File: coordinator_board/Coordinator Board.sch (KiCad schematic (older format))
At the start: 26 parts, among them J1 Conn_01x04, J2 Conn_01x04, J3 Conn_01x04, J4 Conn_01x04, P4 SERIAL, SW1 Switch_SPDT_x2, SW2 Switch_DPST, U0 10118194, U1 LM3671, U3 ESP-12E, U4 DIY-OLED-0.96, U5 SF303GJ26, U6 CD40109B, U7 CD40109B

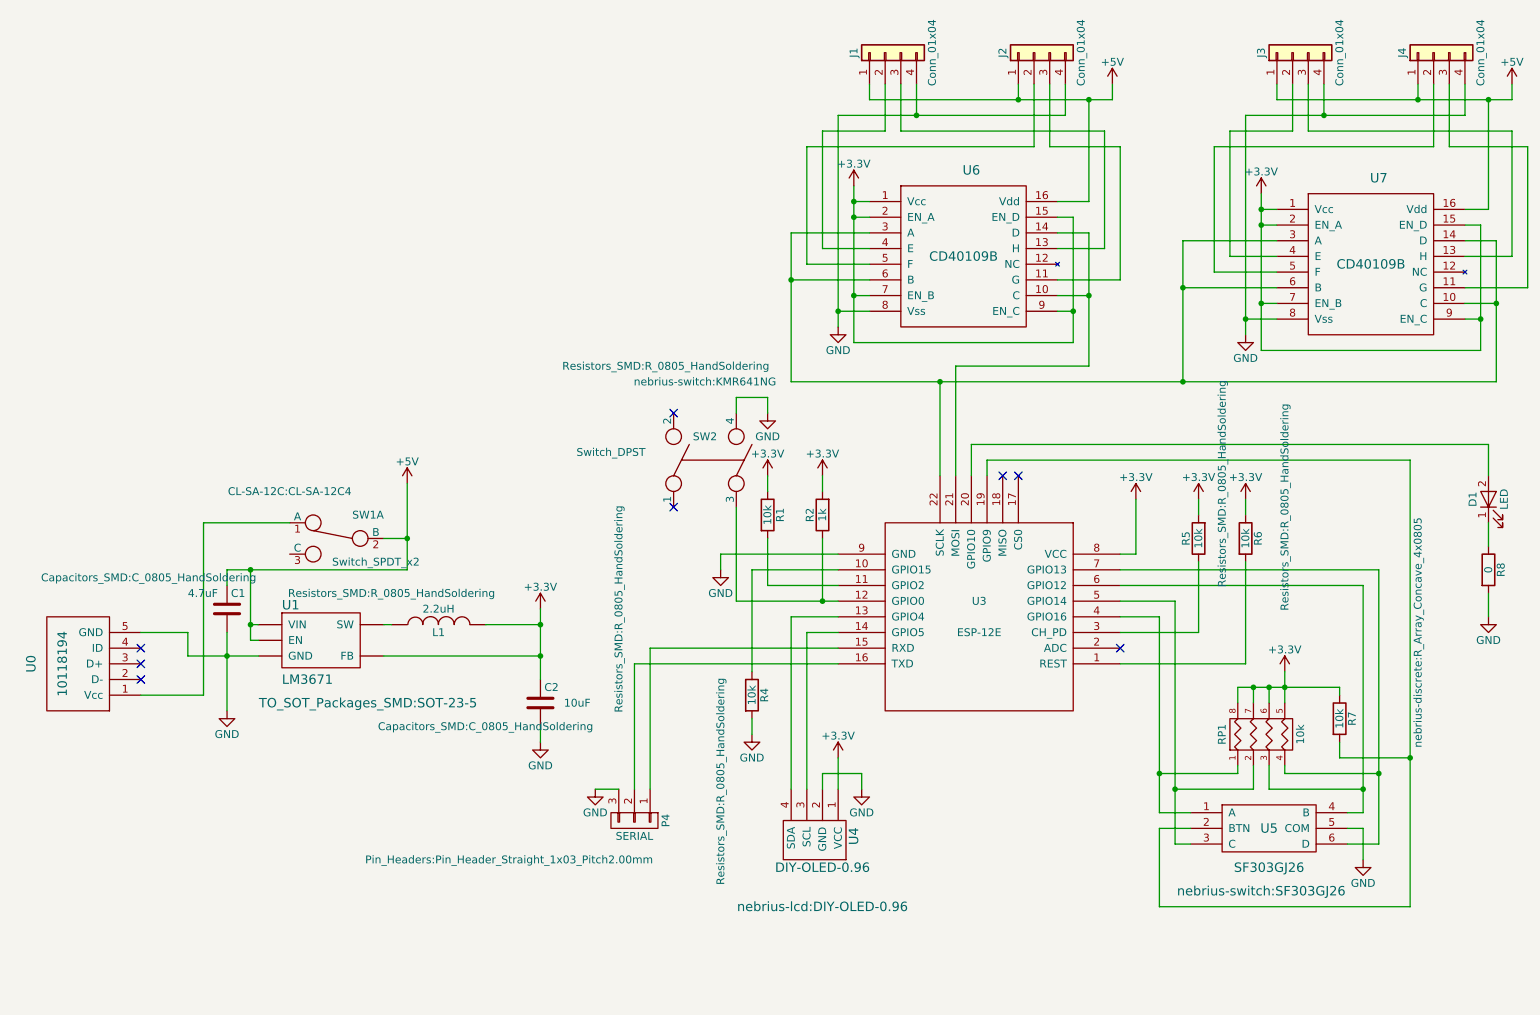
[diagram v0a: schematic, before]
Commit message: Finished most of the layout
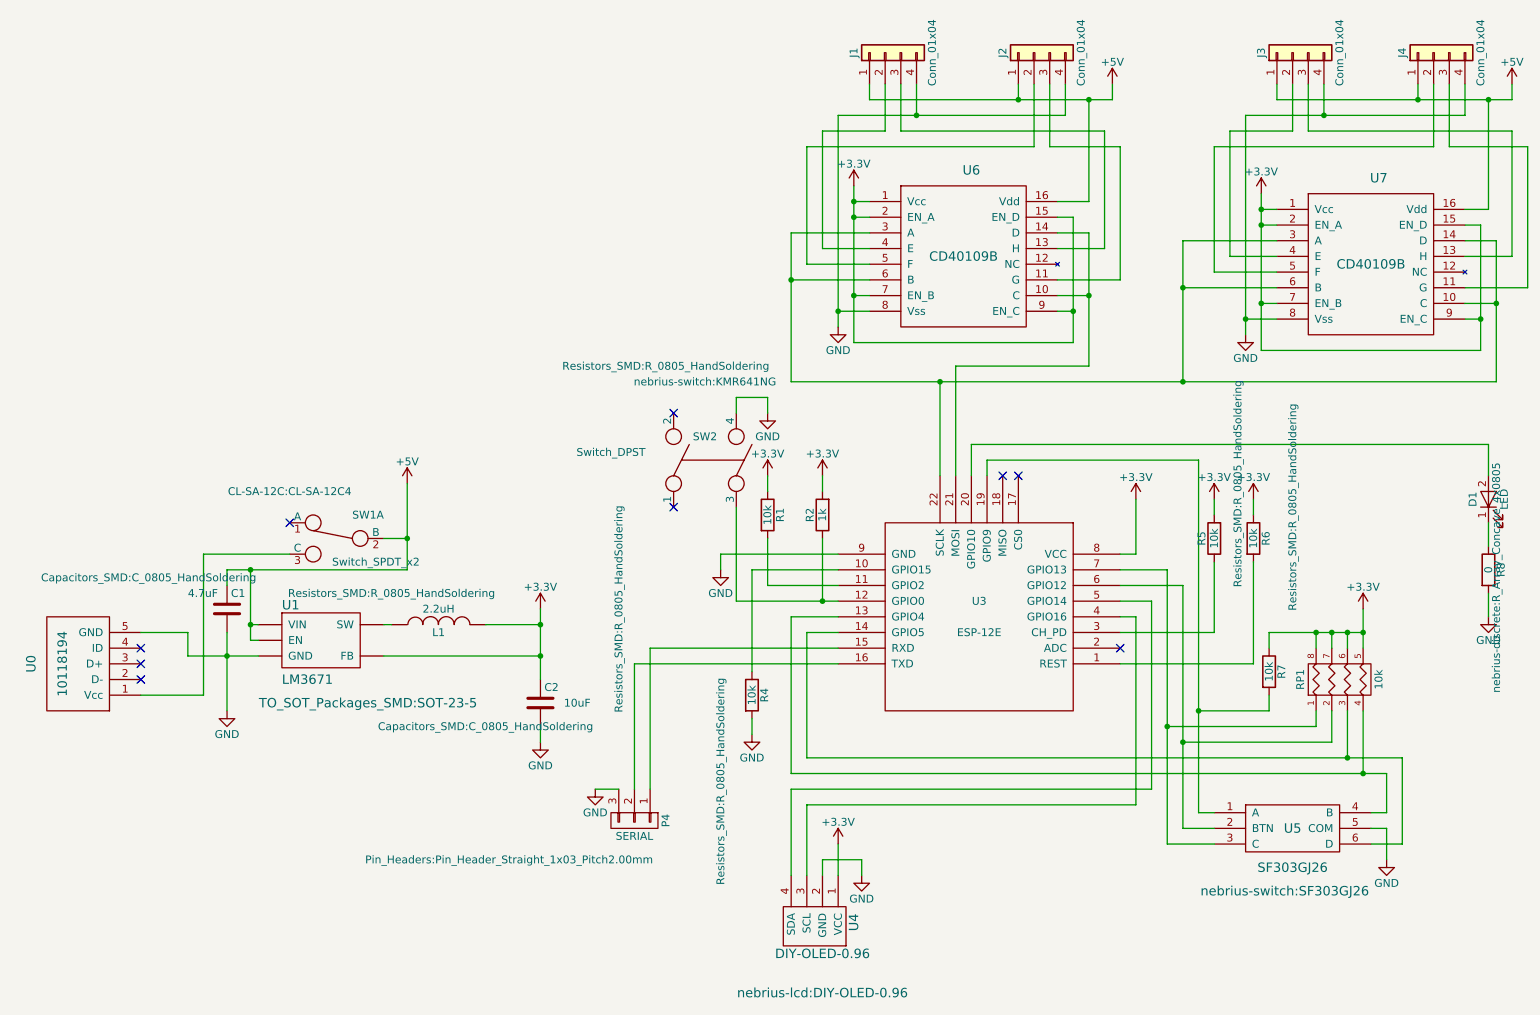
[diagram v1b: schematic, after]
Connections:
- net at SW1.1 (A): no longer U0.1 (Vcc)
- net at SW1.3 (C): now also U0.1 (Vcc)
- net at U3.13 (GPIO4): now also RP1.4 (P4), U5.4 (B); no longer U4.4 (SDA)
- net at U3.14 (GPIO5): now also RP1.3 (P3), U5.6 (D); no longer U4.3 (SCL)
- net at R7.2, U3.19 (GPIO9): now also U5.1 (A); no longer U5.2 (BTN)
- new net: U3.4 (GPIO16), U4.3 (SCL)
- new net: U3.5 (GPIO14), U4.4 (SDA)
- new net: RP1.2 (P2), U3.6 (GPIO12), U5.2 (BTN)
- new net: RP1.1 (P1), U3.7 (GPIO13), U5.3 (C)
- no-connect marks 8 -> 9
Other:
- moved on the sheet: R5, R6, R7, RP1, U4, U5
